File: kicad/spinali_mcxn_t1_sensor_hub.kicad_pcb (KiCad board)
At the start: 6 copper layers, 36.6 x 46 mm, 204 parts, among them J1 5055780421, J10 SDO, J11 CKO, J12 GND, J2 USB4105-GF-A, J3 CAN0A, J4 CAN0B, J5 Debug, J6 CAN1A, J7 CAN1B, J8 DF40TC(3.0)-50DP-0.4V(51), J9 DF40TC(3.0)-50DP-0.4V(51), Q1 BUK6D56-60EX, SW1 SW_SPST, U1 LM74700, U10 BMM350, U11 BMP581, U12 TJA1462ATK, U13 TJA1462ATK, U14 SK9822-EC20, U15 TJA1103AHN, U2 NX5P3363UKZ, U3 LM5160DNTJ, U4 NX5P3363UKZ, U5 MIC5504-1.8YMT, U6 MPM3811GG-Z, U7 MCXN947VDFT, U8 PCMF1USB3SZ, U9 ICM-45686, Y1 24MHz, Y2 32.768kHz, Y3 25MHz

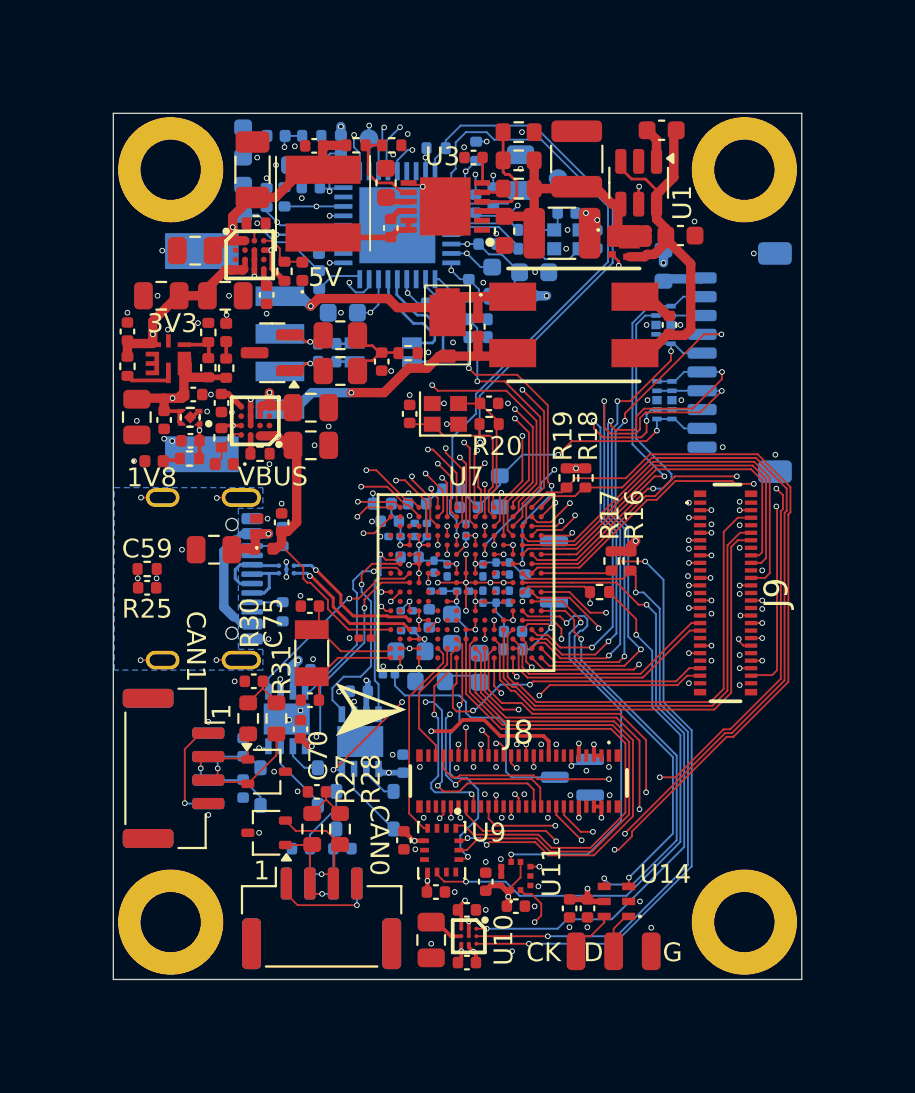
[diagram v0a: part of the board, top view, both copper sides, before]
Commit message: Updated layout
Made edge cut dimensions easy to work with values.
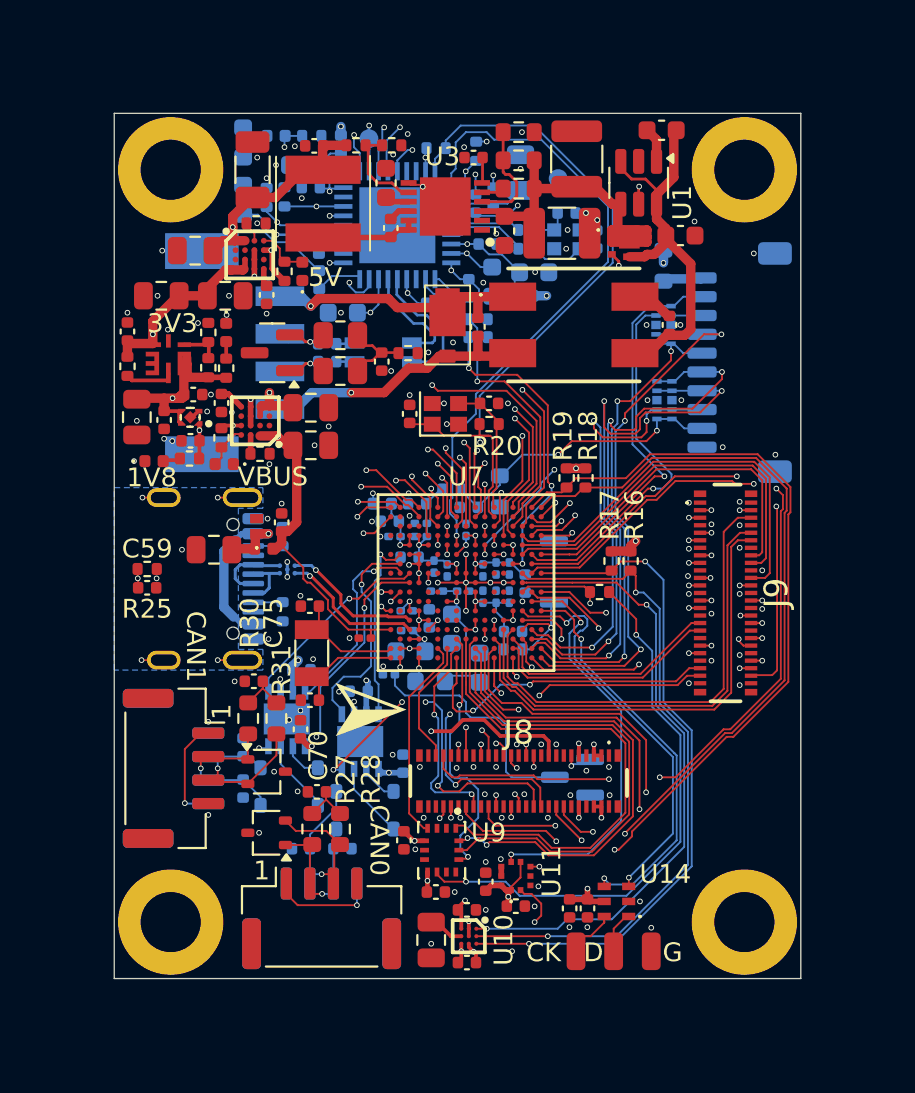
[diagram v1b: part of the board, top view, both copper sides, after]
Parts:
- moved J2 0.06 mm to (85.9, 100.7)
- moved U8 0.05 mm to (91.4, 100.2)
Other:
- board size 36.6 x 46 mm -> 36.5 x 46 mm
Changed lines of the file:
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@@
 	(footprint "TVS:PESD1USB3BCX"
 		(layer "B.Cu")
-		(at 91.35 100.2 -90)
+		(at 91.4 100.2 -90)
 		(descr "WLCSP5_2-1-2")
 		(tags "Diode")
@@
 	(footprint "Connector_USB:USB_C_Receptacle_GCT_USB4105-xx-A_16P_TopMnt_Horizontal"
 		(layer "B.Cu")
-		(at 85.85 100.7 90)
+		(at 85.91 100.7 90)
 		(descr "USB 2.0 Type C Receptacle, GCT, 16P, top mounted, horizontal, 5A: https://gct.co/files/drawings/usb4105.pdf")
 		(tags "USB C Type-C Receptacle SMD USB 2.0 16P 16C USB4105-15-A USB4105-15-A-060 USB4105-15-A-120 USB4105-GF-A USB4105-GF-A-060 USB4105-GF-A-120")
@@
 	)
 	(gr_rect
-		(start 82.15 75.95)
-		(end 118.75 122)
+		(start 82.2 75.95)
+		(end 118.7 121.95)
 		(stroke
 			(width 0.05)
@@
 	)
 	(via
-		(at 91.35 99.8)
+		(at 91.4 99.8)
 		(size 0.3)
 		(drill 0.2)
@@
 	)
 	(via
-		(at 91.35 100.6)
+		(at 91.4 100.6)
 		(size 0.3)
 		(drill 0.2)
@@
 	)
 	(segment
-		(start 91.35 100.2)
-		(end 91.35 99.85)
+		(start 91.4 100.2)
+		(end 91.4 99.85)
 		(width 0.16)
 		(layer "B.Cu")
@@
 	)
 	(segment
-		(start 91.35 99.85)
-		(end 91.35 99.8)
+		(start 91.4 99.85)
+		(end 91.4 99.8)
 		(width 0.16)
 		(layer "B.Cu")
@@
 	)
 	(segment
-		(start 91.35 100.55)
-		(end 91.35 100.6)
+		(start 91.4 100.55)
+		(end 91.4 100.6)
 		(width 0.16)
 		(layer "B.Cu")
@@
 	)
 	(segment
-		(start 91.35 100.2)
-		(end 91.35 100.55)
+		(start 91.4 100.2)
+		(end 91.4 100.55)
 		(width 0.16)
 		(layer "B.Cu")
@@
 	)
 	(segment
-		(start 88.55 102.730406)
-		(end 88.922297 103.102703)
+		(start 89.59 98.3)
+		(end 88.979594 98.3)
 		(width 0.3)
 		(layer "B.Cu")
@@
 	)
 	(segment
-		(start 89.527297 103.102703)
-		(end 89.53 103.1)
-		(width 0.3)
+		(start 88.025 102.205406)
+		(end 88.025 99.230001)
+		(width 0.5)
 		(layer "B.Cu")
 		(net 22)
 	)
 	(segment
-		(start 88.955001 98.3)
-		(end 88.630001 98.625)
+		(start 88.979594 103.1)
+		(end 89.53 103.1)
 		(width 0.3)
 		(layer "B.Cu")
@@
 	)
 	(segment
-		(start 88.922297 103.102703)
-		(end 89.527297 103.102703)
+		(start 88.61 102.730406)
+		(end 88.979594 103.1)
 		(width 0.3)
 		(layer "B.Cu")
@@
 	)
 	(segment
-		(start 89.53 98.3)
+		(start 89.59 98.3)
 		(end 90.4 98.3)
 		(width 0.5)
@@
 	)
 	(segment
-		(start 88.025 102.205406)
-		(end 88.025 99.230001)
+		(start 88.55 102.730406)
+		(end 88.61 102.730406)
+		(width 0.3)
+		(layer "B.Cu")
+		(net 22)
+	)
+	(segment
+		(start 88.025 99.230001)
+		(end 88.630001 98.625)
 		(width 0.5)
 		(layer "B.Cu")
@@
 	)
 	(segment
-		(start 88.025 99.230001)
+		(start 88.654594 98.625)
 		(end 88.630001 98.625)
-		(width 0.5)
+		(width 0.3)
 		(layer "B.Cu")
 		(net 22)
 	)
 	(segment
-		(start 89.53 98.3)
-		(end 88.955001 98.3)
+		(start 88.979594 98.3)
+		(end 88.654594 98.625)
 		(width 0.3)
 		(layer "B.Cu")
@@
 	)
 	(segment
-		(start 87.67 96.38)
-		(end 88.955 96.38)
-		(width 0.1)
-		(layer "F.Cu")
-		(net 24)
-	)
-	(segment
-		(start 83.605 105.02)
-		(end 83.6 105.025)
-		(width 0.1)
-		(layer "F.Cu")
-		(net 24)
-	)
-	(segment
 		(start 83.47 101.175)
 		(end 83.47 100.695)
@@
 	)
 	(segment
-		(start 84.775 105.02)
-		(end 83.605 105.02)
+		(start 87.7 96.38)
+		(end 88.955 96.38)
 		(width 0.1)
 		(layer "F.Cu")
@@
 	)
 	(segment
-		(start 87.65 96.4)
-		(end 87.67 96.38)
+		(start 83.47 100.695)
+		(end 83.45 100.675)
 		(width 0.1)
 		(layer "F.Cu")
@@
 	)
 	(segment
-		(start 83.47 100.695)
+		(start 83.44 100.665)
 		(end 83.45 100.675)
 		(width 0.1)
@@
 	)
 	(segment
-		(start 83.44 100.665)
-		(end 83.45 100.675)
+		(start 83.7 96.38)
+		(end 84.775 96.38)
 		(width 0.1)
 		(layer "F.Cu")
@@
 	)
 	(segment
-		(start 83.62 96.38)
-		(end 84.775 96.38)
+		(start 83.65 105.02)
+		(end 84.775 105.02)
 		(width 0.1)
 		(layer "F.Cu")
@@
 	)
 	(segment
-		(start 87.63 105.02)
+		(start 87.7 105.02)
 		(end 88.955 105.02)
 		(width 0.1)
@@
 	)
 	(via
-		(at 83.62 96.38)
+		(at 83.7 96.38)
 		(size 0.3)
 		(drill 0.2)
@@
 	)
 	(via
-		(at 87.63 105.02)
+		(at 87.7 105.02)
 		(size 0.3)
 		(drill 0.2)
@@
 	)
 	(via
-		(at 83.6 105.025)
+		(at 83.65 105.02)
 		(size 0.3)
 		(drill 0.2)
@@
 	)
 	(via
-		(at 87.65 96.4)
+		(at 87.7 96.38)
 		(size 0.3)
 		(drill 0.2)
@@
 	)
 	(segment
-		(start 89.53 100.95)
-		(end 88.89 100.95)
-		(width 0.16)
-		(layer "B.Cu")
-		(net 231)
-	)
-	(segment
-		(start 89.53 99.95)
-		(end 89.58 100)
+		(start 88.63 100.21)
+		(end 88.89 99.95)
 		(width 0.16)
 		(layer "B.Cu")
@@
 	)
 	(segment
-		(start 88.63 100.69)
-		(end 88.63 100.21)
+		(start 89.53 100.95)
+		(end 88.89 100.95)
 		(width 0.16)
 		(layer "B.Cu")
@@
 	)
 	(segment
-		(start 88.63 100.21)
-		(end 88.89 99.95)
+		(start 89.58 100)
+		(end 91 100)
 		(width 0.16)
 		(layer "B.Cu")
@@
 	)
 	(segment
-		(start 88.89 99.95)
-		(end 89.53 99.95)
+		(start 88.63 100.69)
+		(end 88.63 100.21)
 		(width 0.16)
 		(layer "B.Cu")
@@
 	)
 	(segment
-		(start 89.58 100)
-		(end 90.95 100)
+		(start 89.53 99.95)
+		(end 89.58 100)
 		(width 0.16)
 		(layer "B.Cu")
@@
 	)
 	(segment
-		(start 90.17 101.45)
-		(end 90.44 101.18)
-		(width 0.16)
-		(layer "B.Cu")
-		(net 232)
-	)
-	(segment
-		(start 90.44 101.18)
-		(end 90.44 100.41)
+		(start 88.89 99.95)
+		(end 89.53 99.95)
 		(width 0.16)
 		(layer "B.Cu")
-		(net 232)
+		(net 231)
 	)
 	(segment
-		(start 90.36 100.41)
-		(end 90.916532 100.41)
+		(start 89.53 100.45)
+		(end 89.57 100.41)
 		(width 0.16)
 		(layer "B.Cu")
@@
 	)
 	(segment
-		(start 89.57 100.41)
-		(end 90.36 100.41)
+		(start 90.17 101.45)
+		(end 90.44 101.18)
 		(width 0.16)
 		(layer "B.Cu")
@@
 	)
 	(segment
-		(start 90.916532 100.41)
-		(end 90.928266 100.421734)
+		(start 89.57 100.41)
+		(end 90.99 100.41)
 		(width 0.16)
 		(layer "B.Cu")
@@
 	)
 	(segment
-		(start 89.53 100.45)
-		(end 89.57 100.41)
+		(start 90.44 101.18)
+		(end 90.44 100.41)
 		(width 0.16)
 		(layer "B.Cu")
@@
 	)
 	(segment
-		(start 92.45 100.4)
-		(end 91.75 100.4)
+		(start 92.6 100.55)
+		(end 92.45 100.4)
 		(width 0.16)
 		(layer "B.Cu")
@@
 	)
 	(segment
-		(start 92.6 100.55)
-		(end 92.45 100.4)
+		(start 92.45 100.4)
+		(end 91.8 100.4)
 		(width 0.16)
 		(layer "B.Cu")
@@
 	(segment
 		(start 92.6764 99.99)
-		(end 91.76 99.99)
+		(end 91.81 99.99)
 		(width 0.16)
 		(layer "B.Cu")
@@
 	)
 	(segment
-		(start 92.9182 100.2318)
-		(end 92.6764 99.99)
+		(start 91.81 99.99)
+		(end 91.8 100)
 		(width 0.16)
 		(layer "B.Cu")
@@
 	)
 	(segment
-		(start 91.76 99.99)
-		(end 91.75 100)
+		(start 92.9182 100.2318)
+		(end 92.6764 99.99)
 		(width 0.16)
 		(layer "B.Cu")
